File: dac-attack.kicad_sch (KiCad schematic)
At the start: 57 parts, among them J1 BOARD, J2 BOARD, J3 BOARD, J4 ANALOG, J5 DIGITAL, J6 USER, J7 BTN, U1 CS8416-xZZ, U2 PCM5100, U3 SD6210A, U4 XC6206P332MR, U5 XC6206P332MR

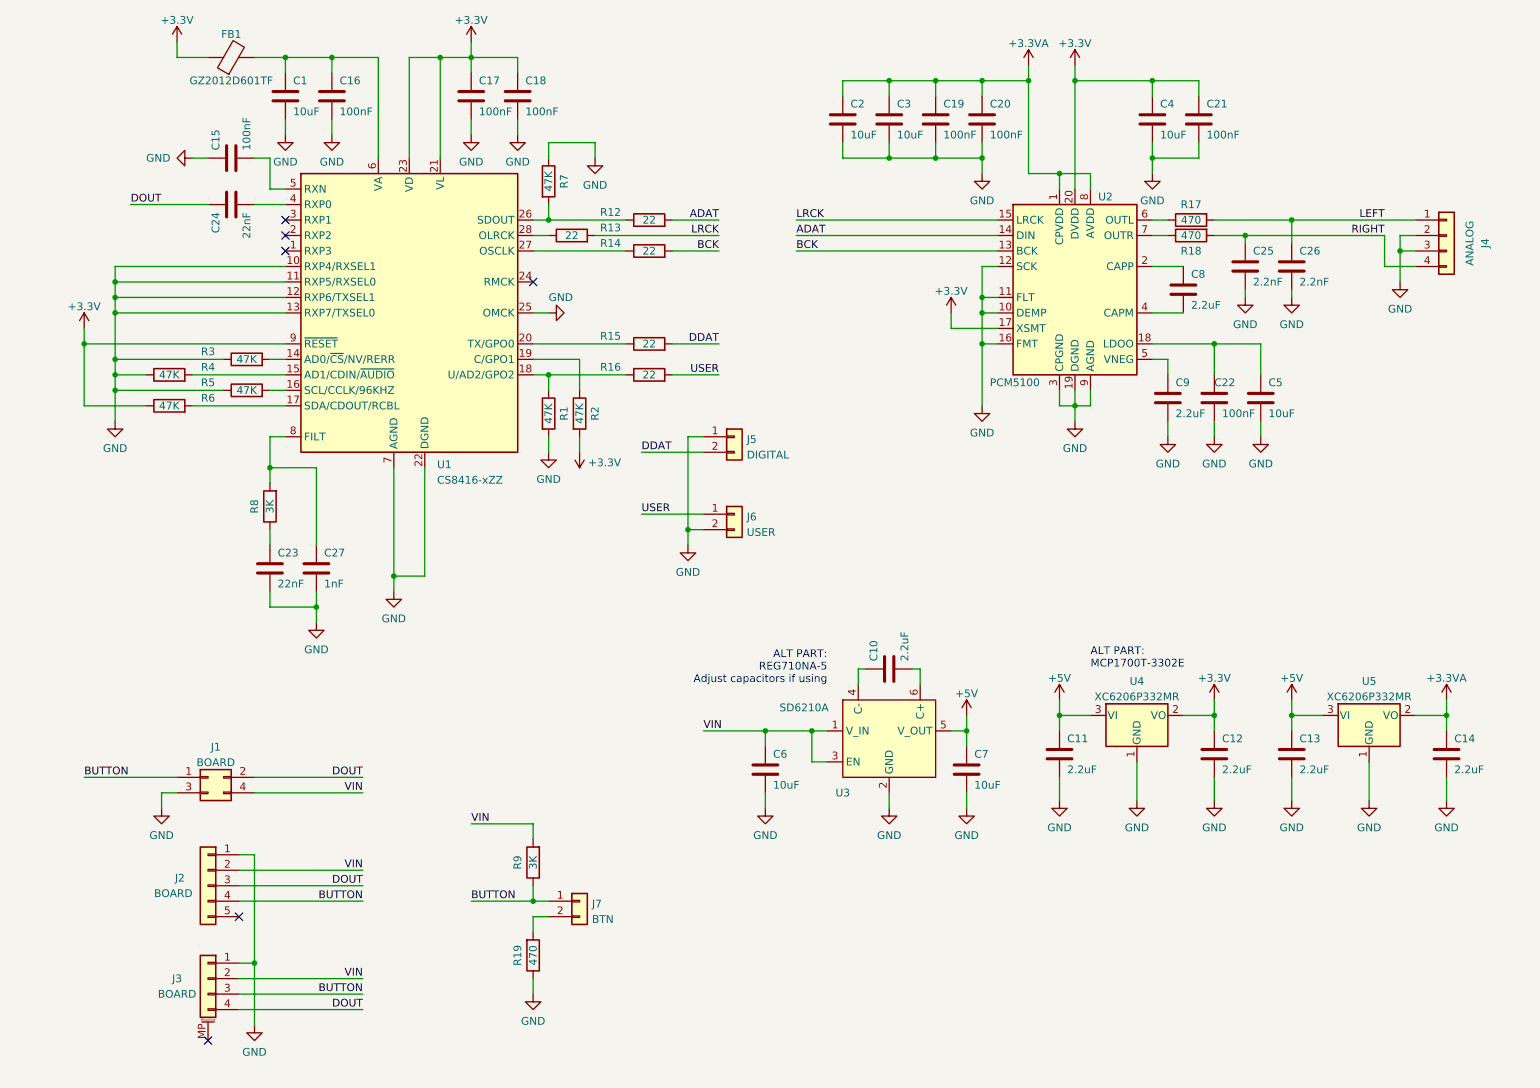
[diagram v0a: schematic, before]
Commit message: Initial work on revision 2023b.
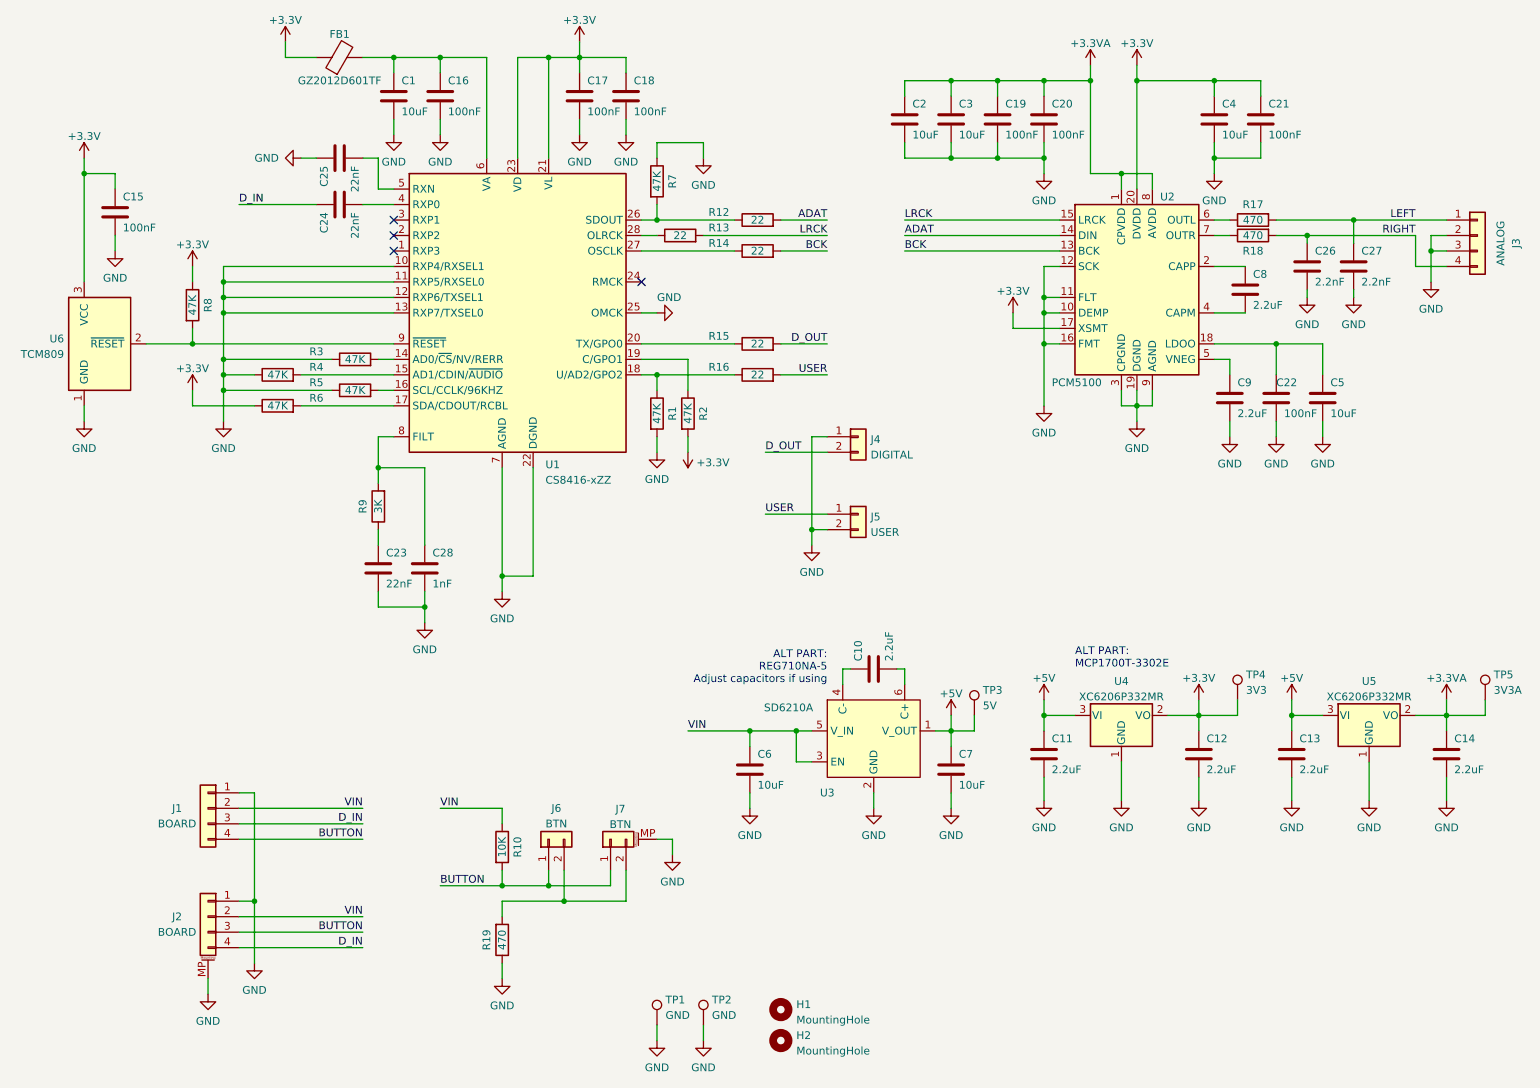
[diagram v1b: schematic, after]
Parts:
- removed J1: BOARD, Connector_PinSocket_2.54mm:PinSocket_2x02_P2.54mm_Vertical, symbol Connector_Generic:Conn_02x02_Odd_Even
- removed J2: BOARD, Connector_PinSocket_2.54mm:PinSocket_1x05_P2.54mm_Vertical, symbol Connector_Generic:Conn_01x05
- removed R9: 3K, Resistor_SMD:R_0603_1608Metric, symbol Device:R
- added C25: 22nF, Capacitor_SMD:C_0402_1005Metric, symbol Device:C
- added H1, H2: MountingHole, MountingHole:MountingHole_3.2mm_M3, symbol Mechanical:MountingHole
- added J1: BOARD, Connector_PinHeader_2.54mm:PinHeader_1x04_P2.54mm_Vertical, symbol Connector_Generic:Conn_01x04
- added J7: BTN, Connector_JST:JST_SH_SM02B-SRSS-TB_1x02-1MP_P1.00mm_Horizontal, symbol Connector_Generic_MountingPin:Conn_01x02_MountingPin
- added R10: 10K, Resistor_SMD:R_0402_1005Metric, symbol Device:R
- added R8: 47K, Resistor_SMD:R_0402_1005Metric, symbol Device:R
- added TP1, TP2: GND, TestPoint:TestPoint_Keystone_5000-5004_Miniature, symbol Connector:TestPoint
- added TP3: 5V, TestPoint:TestPoint_Pad_D1.0mm, symbol Connector:TestPoint
- added TP4: 3V3, TestPoint:TestPoint_Pad_D1.0mm, symbol Connector:TestPoint
- added TP5: 3V3A, TestPoint:TestPoint_Pad_D1.0mm, symbol Connector:TestPoint
- added U6: TCM809, Package_TO_SOT_SMD:SOT-23, symbol Power_Supervisor:TCM809
- J5: renamed from J6; footprint Connector_PinHeader_2.54mm:PinHeader_1x02_P2.54mm_Horizontal -> Connector_PinHeader_2.54mm:PinHeader_1x02_P2.54mm_Vertical
- renumbered C25 to C26, C26 to C27, C27 to C28, J3 to J2, J4 to J3, J5 to J4, J7 to J6, R8 to R9
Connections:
- net +3.3VA: now also TP5.1
- net +3V3: now also C15.1, R8.1, TP4.1, U6.3 (VCC); no longer U1.9 (~{RESET})
- net +5V: now also U3.1 (V_OUT), TP3.1; no longer U3.5 (V_OUT)
- net BUTTON: now also J1.4 (Pin_4), J7.1 (Pin_1), R10.2
- net GND: now also C15.2, J2.MP (MountPin), C25.1, J1.1 (Pin_1), J7.MP (MountPin), TP1.1, TP2.1, U6.1 (GND); no longer C15.1
- net VIN: now also U3.5 (V_IN), J1.2 (Pin_2), R10.1; no longer U3.1 (V_IN)
- net at J6.2 (Pin_2), R19.2: now also J7.2 (Pin_2)
- net at U1.5 (RXN): now also C25.2; no longer C15.2
- net DDAT renamed D_OUT
- net DOUT renamed D_IN
- net D_IN: now also J1.3 (Pin_3)
- new net: R8.2, U1.9 (~{RESET}), U6.2 (~{RESET})
- no-connect marks 6 -> 4
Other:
- moved on the sheet: C1, C10, C11, C12, C15, C16, C17, C18, C19, C2, C20, C21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
